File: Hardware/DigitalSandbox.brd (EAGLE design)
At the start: 109.2 x 76.2 mm, 80 parts, among them J1 AVR_SPI_PRG_6NS, Q1 MOSFET-N, Q2 MOSFET-P, U1 MCP73831, U2 ATMEGA328, U3 C2031N-1A2-B10K-GP, U4 MCP9700, U5 FT232RLSSOP, U6 LIGHTSENSORALS, U7 V_REG_LDOSMD, U8 LMV358, U9 MIC9.7MM, X1 USB-SMD-NS, Y1 8MHz

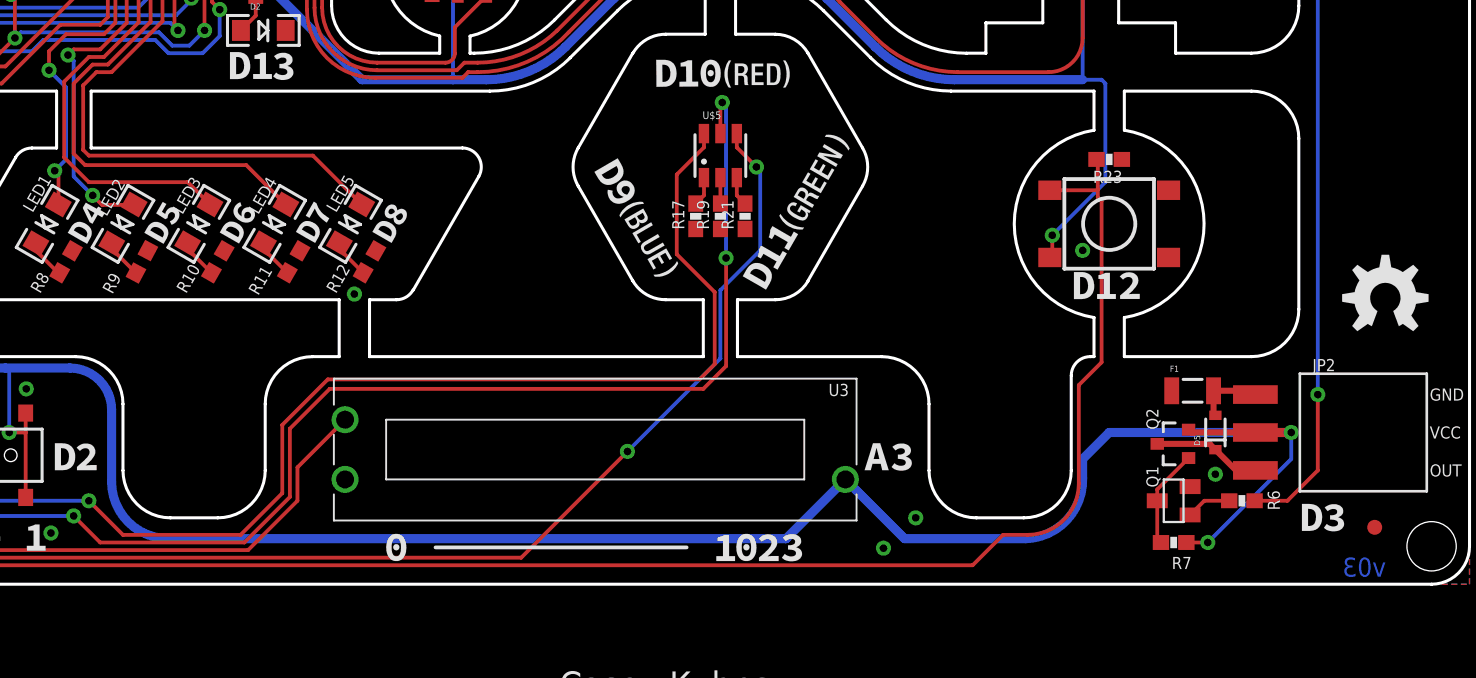
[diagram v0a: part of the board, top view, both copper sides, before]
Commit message: added Rev number
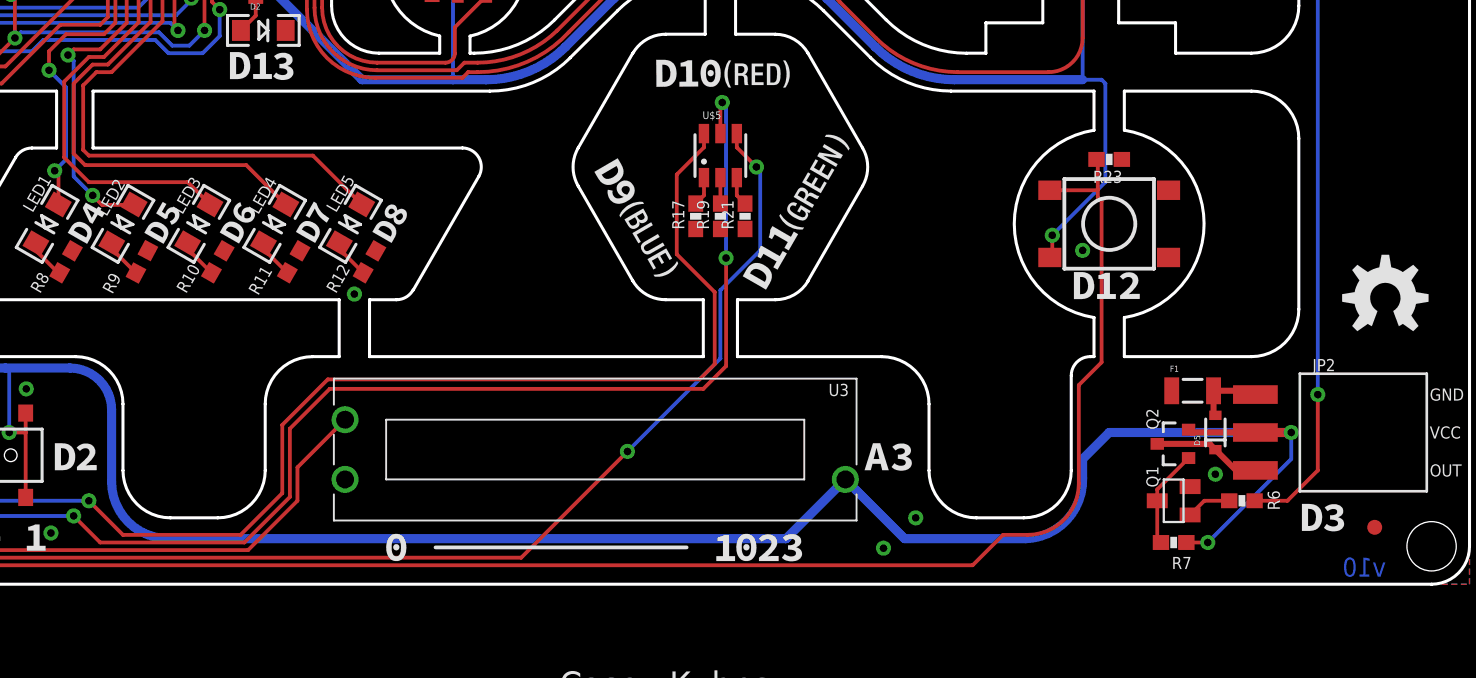
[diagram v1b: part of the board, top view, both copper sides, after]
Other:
- outline, holes or cut-outs redrawn
- board text added: "v10"
- board text removed: "v03"
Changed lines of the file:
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@@
 <setting verticaltext="up"/>
 </settings>
-<grid distance="10" unitdist="mil" unit="mil" style="lines" multiple="1" display="yes" altdistance="0.005" altunitdist="inch" altunit="inch"/>
+<grid distance="5" unitdist="mil" unit="mil" style="lines" multiple="1" display="yes" altdistance="0.005" altunitdist="inch" altunit="inch"/>
 <layers>
 <layer number="1" name="Top" color="4" fill="1" visible="yes" active="yes"/>
@@
 <wire x1="33.528" y1="19.05" x2="8.5598" y2="19.05" width="0.2032" layer="20"/>
 <wire x1="42.8752" y1="27.305" x2="38.481" y2="19.685" width="0.2032" layer="20"/>
-<wire x1="16.9164" y1="29.21" x2="41.783" y2="29.21" width="0.2032" layer="20"/>
+<wire x1="17.0434" y1="29.21" x2="41.783" y2="29.21" width="0.2032" layer="20"/>
 <wire x1="48.9966" y1="35.2552" x2="52.1716" y2="38.4048" width="0.2032" layer="20"/>
 <wire x1="42.5704" y1="35.56" x2="42.291" y2="35.56" width="0.2032" layer="20"/>
@@
 <wire x1="53.1876" y1="20.32" x2="55.3973875" y2="19.0522875" width="0.2032" layer="20" curve="60.257051"/>
 <wire x1="53.1876" y1="20.32" x2="49.53" y2="26.67" width="0.2032" layer="20"/>
-<wire x1="16.9164" y1="33.02" x2="43.6118" y2="33.02" width="0.2032" layer="20"/>
+<wire x1="17.0434" y1="33.02" x2="43.6118" y2="33.02" width="0.2032" layer="20"/>
 <wire x1="58.039" y1="43.18" x2="56.4896" y2="43.18" width="0.2032" layer="20"/>
 <wire x1="86.106" y1="33.02" x2="94.615" y2="33.02" width="0.2032" layer="20"/>
@@
 <wire x1="83.82" y1="15.24" x2="82.55" y2="13.97" width="0.2032" layer="20" curve="90"/>
 <wire x1="14.605" y1="29.21" x2="14.605" y2="33.02" width="0.2032" layer="20"/>
-<wire x1="16.9164" y1="33.02" x2="16.9164" y2="29.21" width="0.2032" layer="20"/>
+<wire x1="17.0434" y1="33.02" x2="17.0434" y2="29.21" width="0.2032" layer="20"/>
 <wire x1="60.071" y1="67.056" x2="60.071" y2="61.7728" width="0.2032" layer="20"/>
 <wire x1="58.039" y1="61.7728" x2="58.039" y2="67.056" width="0.2032" layer="20"/>
@@
 <wire x1="0" y1="2.54" x2="2.54" y2="0" width="0.2032" layer="20" curve="90"/>
 <text x="48.26" y="-7.62" size="1.778" layer="25">Casey Kuhns</text>
-<text x="103.632" y="0.508" size="1.27" layer="16" font="vector" ratio="20" rot="MR0">v03</text>
+<text x="103.632" y="0.508" size="1.27" layer="16" font="vector" ratio="20" rot="MR0">v10</text>
 <polygon width="0.001" layer="21">
 <vertex x="41.0694" y="68.9322"/>
@@
 </class>
 </classes>
-<designrules name="default">
+<designrules name="SparkFun-2-layer">
 <description language="en">&lt;b&gt;EAGLE Design Rules&lt;/b&gt;
 &lt;p&gt;
@@
 <param name="mdViaViaSameLayer" value="8mil"/>
 <param name="mnLayersViaInSmd" value="2"/>
-<param name="mdCopperDimension" value="10mil"/>
+<param name="mdCopperDimension" value="8mil"/>
 <param name="mdDrill" value="8mil"/>
 <param name="mdSmdStop" value="0mil"/>
-<param name="msWidth" value="6mil"/>
+<param name="msWidth" value="7mil"/>
 <param name="msDrill" value="15mil"/>
 <param name="msMicroVia" value="9.99mm"/>
@@
 <param name="dpGapFactor" value="2.5"/>
 <param name="checkGrid" value="0"/>
-<param name="checkAngle" value="1"/>
+<param name="checkAngle" value="0"/>
 <param name="checkFont" value="1"/>
 <param name="checkRestrict" value="1"/>
